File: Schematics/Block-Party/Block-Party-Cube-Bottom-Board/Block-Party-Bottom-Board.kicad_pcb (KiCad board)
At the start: 2 copper layers, 40 x 40 mm, 10 parts

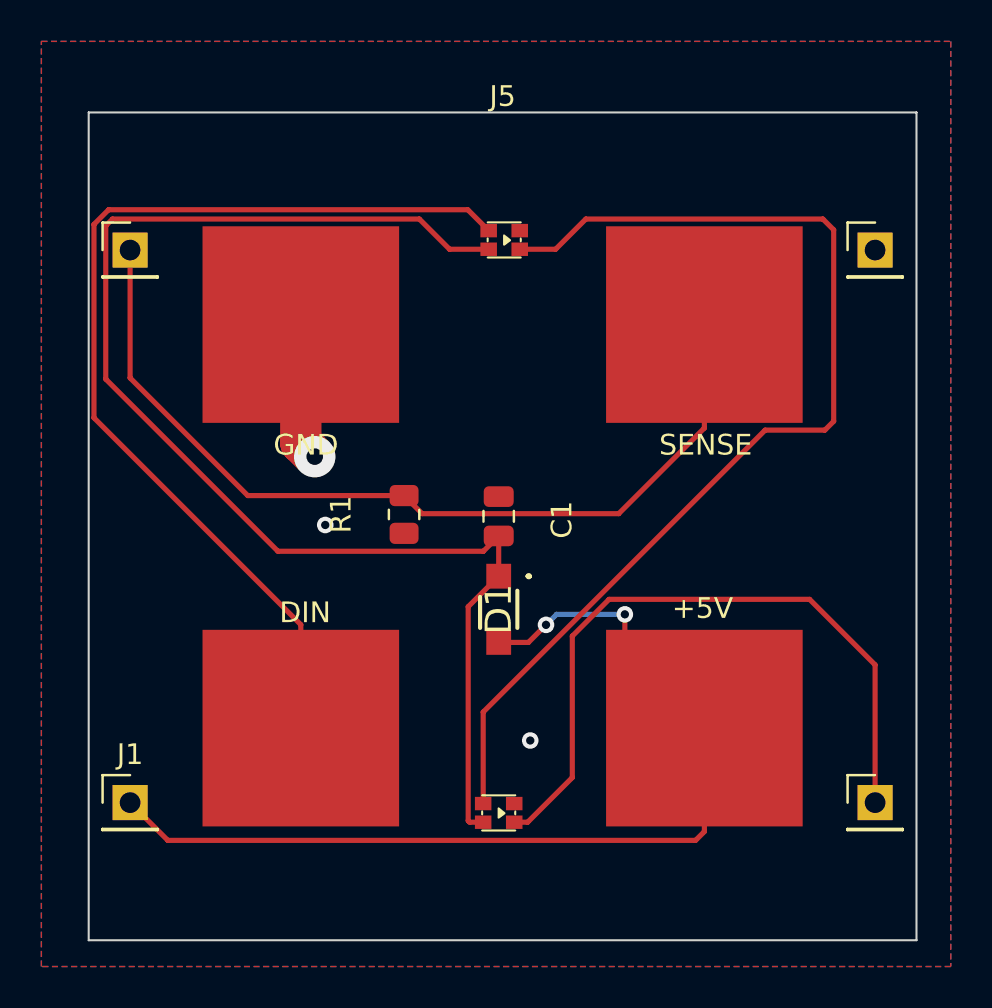
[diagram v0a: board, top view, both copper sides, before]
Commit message: Revision 1.01 of the PCBs
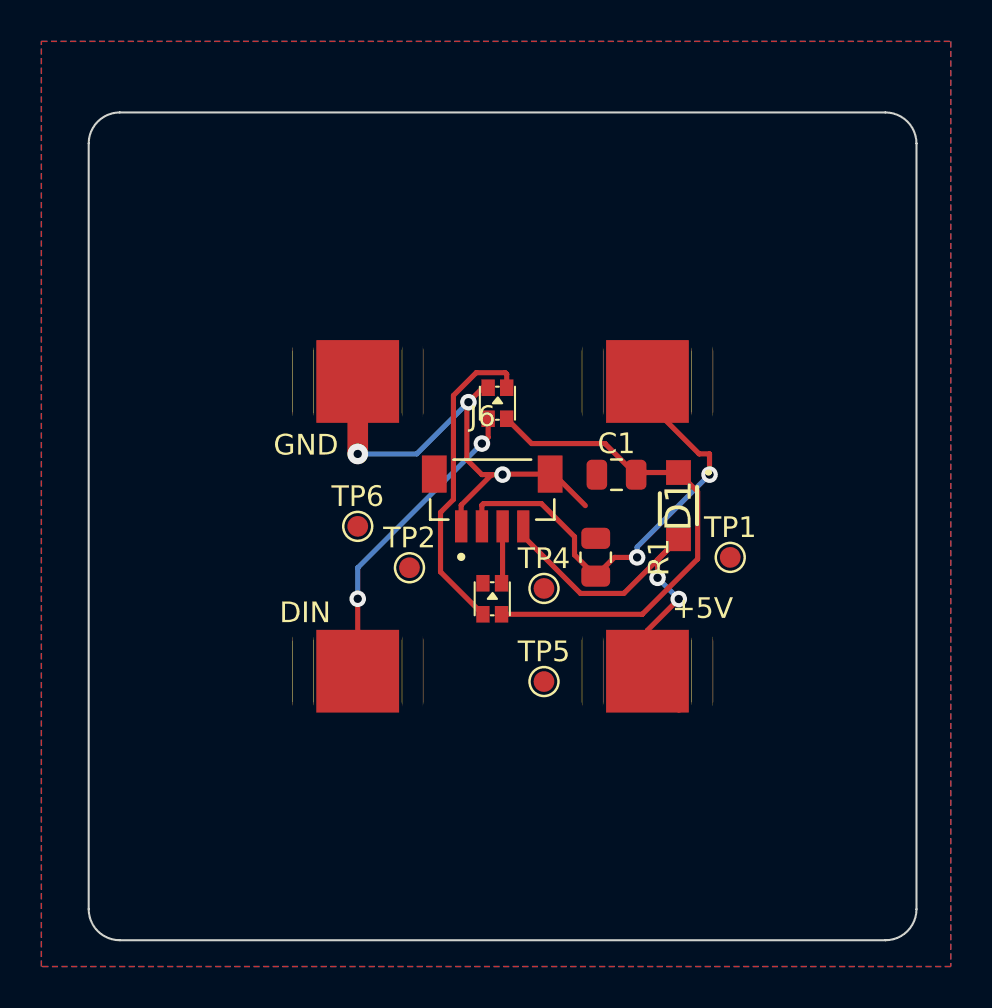
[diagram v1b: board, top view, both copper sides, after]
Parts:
- removed J1, J2, J3, J4: ~, Connector_PinHeader_2.54mm:PinHeader_1x01_P2.54mm_Vertical
- added J6: YTC-A1001LF-04A, adafruit-jst-4328:ADAFRUIT_4328, F.Cu at (159.2, 77.3)
- added TP1: Diode5V, TestPoint:TestPoint_Pad_D1.0mm, F.Cu at (170.7, 80.6)
- added TP2: DODI, TestPoint:TestPoint_Pad_D1.0mm, F.Cu at (155.2, 81.1)
- added TP4: DO, TestPoint:TestPoint_Pad_D1.0mm, F.Cu at (161.7, 82.1)
- added TP5: 5V, TestPoint:TestPoint_Pad_D1.0mm, F.Cu at (161.7, 86.6)
- added TP6: DI, TestPoint:TestPoint_Pad_D1.0mm, F.Cu at (152.7, 79.1)
- moved LED1 10.4 mm to (159.2, 82.6), turned to -90 degrees
- moved D1 10.0 mm to (168.2, 78.1)
- moved R1 9.49 mm to (164.2, 80.6), turned to 90 degrees
- moved LED2 7.90 mm to (159.4, 73.1), turned to -90 degrees
- moved C1 6.04 mm to (165.2, 76.6), turned to 180 degrees
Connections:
- J5 pad 5: (no net) -> unconnected-(J5-HOLE-Pad5)_1
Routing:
- net D5V: track 64.5 -> 24.6 mm
- net Net-(LED1-DI): track 52.4 -> 15.4 mm
- net DIN: track 48.3 -> 15.2 mm, vias 0 -> 2
- net DOUT: track 33.9 -> 2.77 mm
- net +5V: track 47.4 -> 20.6 mm
- net SENSE: track 43.4 -> 22.4 mm, vias 0 -> 2
- net GND: track 6.66 -> 23.5 mm
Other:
- outline, holes or cut-outs redrawn
